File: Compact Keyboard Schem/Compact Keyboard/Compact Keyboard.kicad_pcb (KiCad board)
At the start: 2 copper layers, 105.5 x 115.1 mm, 35 parts, among them J1 MUX+POT, J2 MUX Power, J4 PAM8406 Power, J5 ILI 9341, J6 USB_A, J7 Rotary_Encoder, J8 USB_Host, J9 Jack-DC, Q1 Q_PMOS_GSD, Q2 Q_PMOS_GSD, SW1 SW_Push_LED, SW2 SW_Push, SW3 SW_Push, SW4 SW_Push, SW5 SW_Push

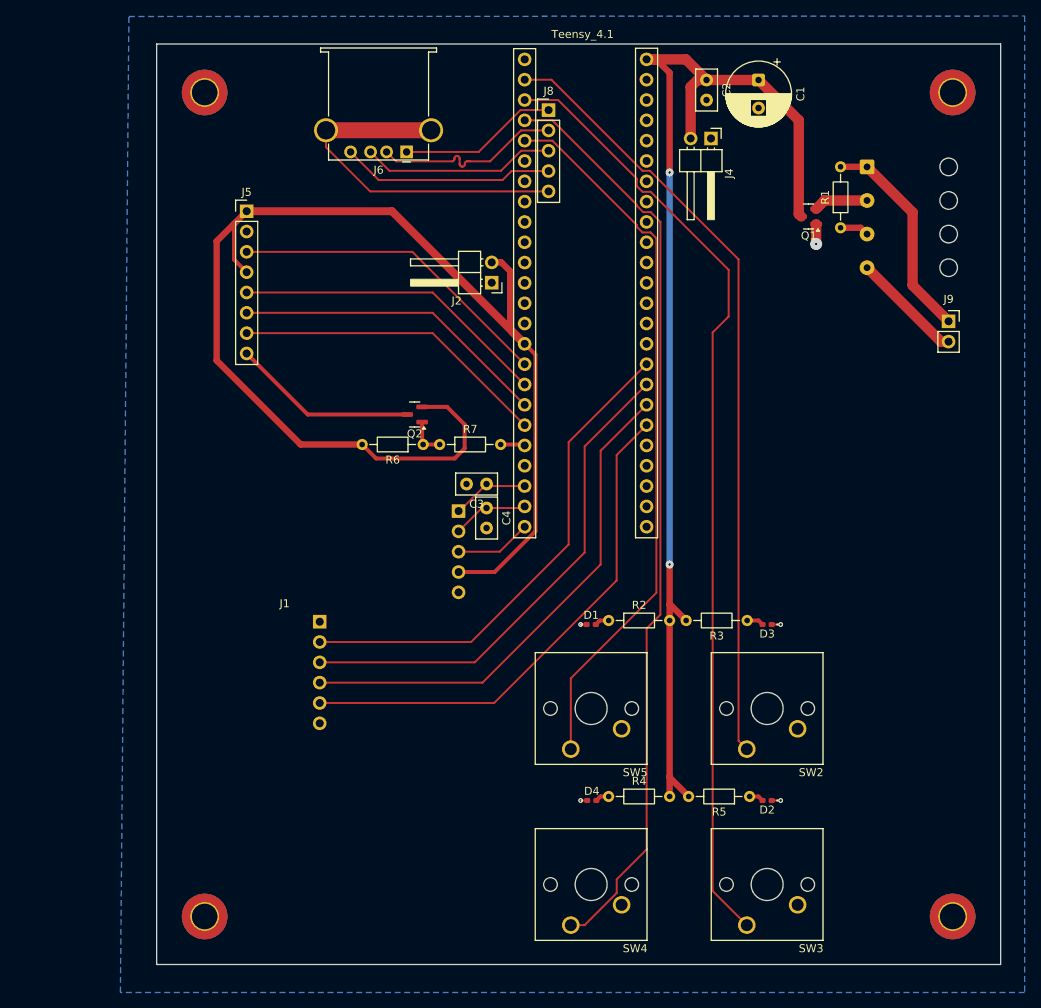
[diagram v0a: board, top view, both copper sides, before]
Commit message: Pushing Update
Latest version after PCB printing
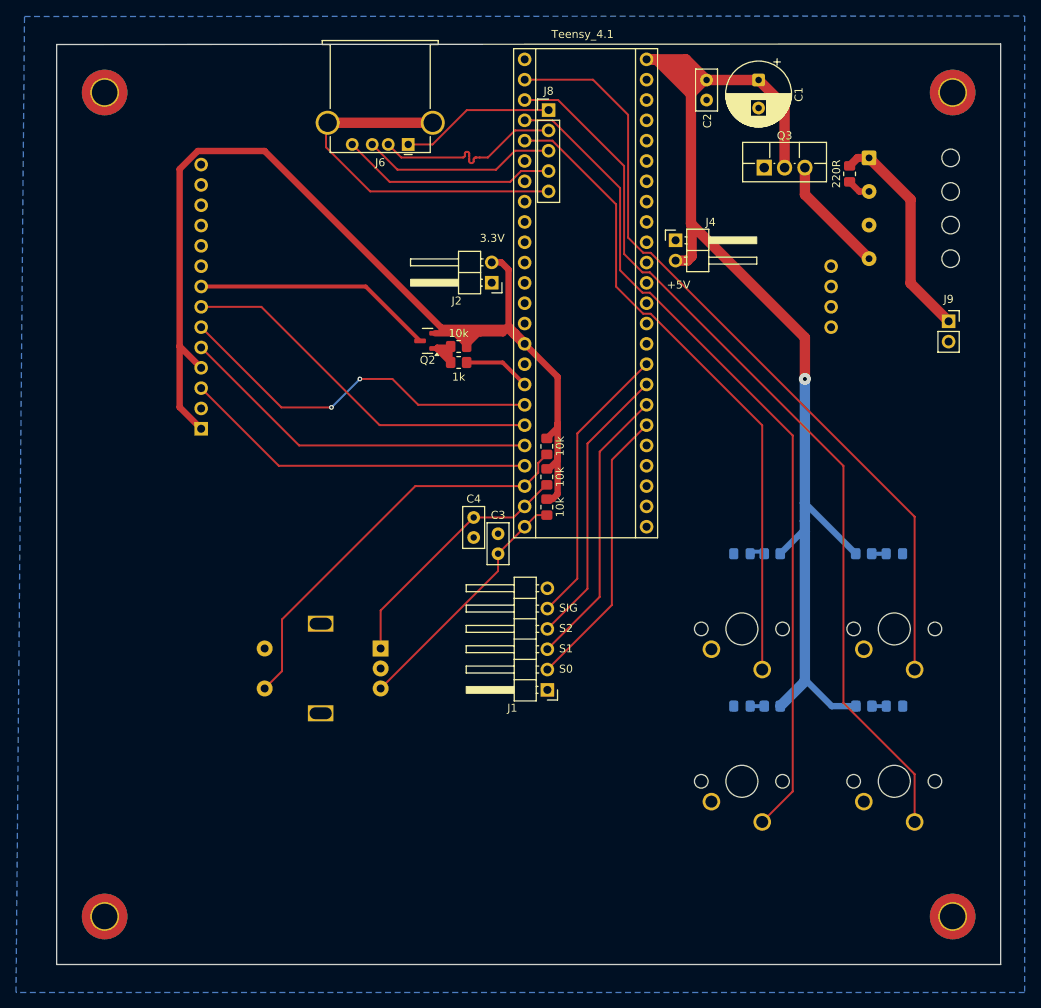
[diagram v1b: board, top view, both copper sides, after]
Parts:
- removed J5: ILI 9341, Connector_PinHeader_2.54mm:PinHeader_1x08_P2.54mm_Vertical
- removed J7: Rotary_Encoder, Connector_PinHeader_2.54mm:PinHeader_1x05_P2.54mm_Horizontal
- removed Q1: Q_PMOS_GSD, Package_TO_SOT_SMD:SOT-23
- added 10k: 10K, Resistor_SMD:R_0805_2012Metric_Pad1.20x1.40mm_HandSolder, F.Cu at (144.3, 83.3)
- added 10k: 10K, Resistor_SMD:R_0805_2012Metric_Pad1.20x1.40mm_HandSolder, F.Cu at (144.3, 79.5)
- added 10k: 10K, Resistor_SMD:R_0805_2012Metric_Pad1.20x1.40mm_HandSolder, F.Cu at (144.3, 75.7)
- added J3: SW_Switch_LED, Connector_Wire:SolderWire-0.25sqmm_1x04_P4.2mm_D0.65mm_OD1.7mm_Relief, B.Cu at (184.5, 39.7)
- added Q3: Q_PMOS_GDS, Package_TO_SOT_THT:TO-220F-3_Vertical, F.Cu at (171.5, 40.9)
- added TFT_ILI1: ~, TOMD:ILI9341_TFT, B.Cu at (140.4, 40.5)
- 10k: renamed from R6; footprint Resistor_THT:R_Axial_DIN0204_L3.6mm_D1.6mm_P7.62mm_Horizontal -> Resistor_SMD:R_0805_2012Metric_Pad1.20x1.40mm_HandSolder
- 1k: renamed from R7; footprint Resistor_THT:R_Axial_DIN0204_L3.6mm_D1.6mm_P7.62mm_Horizontal -> Resistor_SMD:R_0805_2012Metric_Pad1.20x1.40mm_HandSolder
- 220R: renamed from R1; footprint Resistor_THT:R_Axial_DIN0204_L3.6mm_D1.6mm_P7.62mm_Horizontal -> Resistor_SMD:R_0805_2012Metric_Pad1.20x1.40mm_HandSolder
- 220R: renamed from R5; footprint Resistor_THT:R_Axial_DIN0204_L3.6mm_D1.6mm_P7.62mm_Horizontal -> Resistor_SMD:R_0805_2012Metric_Pad1.20x1.40mm_HandSolder; moved to B.Cu
- 220R: renamed from R4; footprint Resistor_THT:R_Axial_DIN0204_L3.6mm_D1.6mm_P7.62mm_Horizontal -> Resistor_SMD:R_0805_2012Metric_Pad1.20x1.40mm_HandSolder; moved to B.Cu
- 220R: renamed from R2; footprint Resistor_THT:R_Axial_DIN0204_L3.6mm_D1.6mm_P7.62mm_Horizontal -> Resistor_SMD:R_0805_2012Metric_Pad1.20x1.40mm_HandSolder; moved to B.Cu
- 220R: renamed from R3; footprint Resistor_THT:R_Axial_DIN0204_L3.6mm_D1.6mm_P7.62mm_Horizontal -> Resistor_SMD:R_0805_2012Metric_Pad1.20x1.40mm_HandSolder; moved to B.Cu
- D1, D2, D3, D4: footprint LED_SMD:LED_0402_1005Metric_Pad0.77x0.64mm_HandSolder -> LED_SMD:LED_0805_2012Metric_Pad1.15x1.40mm_HandSolder; moved to B.Cu
- J1: moved to F.Cu
- SW1: value SW_Push_LED -> RotaryEncoder_Switch_MP; footprint Connector_Wire:SolderWire-0.25sqmm_1x04_P4.2mm_D0.65mm_OD1.7mm_Relief -> Rotary_Encoder:RotaryEncoder_Alps_EC11E-Switch_Vertical_H20mm
- SW2, SW3, SW4, SW5: moved to B.Cu
- moved SW1 85.6 mm to (123.5, 101.0), turned to 180 degrees
- moved D4 39.6 mm to (187.7, 108.2), turned to 180 degrees
- moved D1 38.9 mm to (187.7, 89.2), turned to 180 degrees
- moved 220R 33.9 mm to (183.9, 108.2), turned to 180 degrees
- moved 220R 33.0 mm to (183.9, 89.2), turned to 180 degrees
- moved J1 29.7 mm to (144.3, 106.2)
- moved SW4 27.2 mm to (171.2, 122.7), turned to 0 degrees
- moved SW5 25.9 mm to (171.2, 103.6), turned to 0 degrees
- moved SW3 24.6 mm to (190.2, 122.7), turned to 0 degrees
- moved SW2 23.2 mm to (190.2, 103.6), turned to 0 degrees
- moved J4 13.5 mm to (160.4, 50.0), turned to 0 degrees
- moved 10k 13.0 mm to (133.2, 63.2), turned to 0 degrees
- moved REF** 12.5 mm to (89.0, 31.5)
- moved REF** 12.5 mm to (89.0, 134.5)
- moved D2 12.2 mm to (168.7, 108.2), turned to 0 degrees
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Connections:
- 220R pad 1: Net-(SW1-K) -> Net-(J3-Pin_2)
- 220R pad 2: Net-(J9-Pad1) -> Net-(J3-Pin_1)
- J1 pad 2: /SIG_MUX -> /S0_MUX
- J1 pad 3: /S2_MUX -> /S1_MUX
- J1 pad 4: /S1_MUX -> /S2_MUX
- J1 pad 5: /S0_MUX -> /SIG_MUX
- J9 pad 1: Net-(J9-Pad1) -> Net-(J3-Pin_1)
- Teensy_4.1 pad 16: /ILI_9341/CS_LCD -> unconnected-(Teensy_4.1-24-Pad16)
- Teensy_4.1 pad 17: /ILI_9341/DC_LCD -> /ILI_9341/LED_LCD
- Teensy_4.1 pad 20: /ILI_9341/LED_LCD -> /ILI_9341/DC_LCD
- Teensy_4.1 pad 21: unconnected-(Teensy_4.1-29-Pad21) -> /ILI_9341/CS_LCD
- Teensy_4.1 pad 22: /Rotary_Encoder/CLK_RE -> /Rotary_Encoder/SW_RE
- Teensy_4.1 pad 24: /Rotary_Encoder/SW_RE -> /Rotary_Encoder/CLK_RE
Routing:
- net /Rotary_Encoder/SW_RE: track 9.55 -> 51.9 mm
- net /S0_MUX: track 64.4 -> 35.7 mm
- net /S1_MUX: track 63.6 -> 35.7 mm
- net Net-(J3-Pin_1): track 0.00 -> 27.4 mm
- net /S2_MUX: track 63.0 -> 35.7 mm
- net /SIG_MUX: track 62.7 -> 35.7 mm
- net Net-(J9-Pad1): track 26.8 -> 0.00 mm
- net +3.3V: track 164.9 -> 142.2 mm
- net /Rotary_Encoder/DT_RE: track 9.55 -> 32.0 mm
- net /Rotary_Encoder/CLK_RE: track 9.77 -> 31.0 mm
- net GND: track 20.3 -> 0.00 mm, vias 5 -> 0
- net Net-(J3-Pin_4): track 0.00 -> 14.7 mm
- net /Buttons/BTN3_IN: track 115.8 -> 105.7 mm
- net /Buttons/BTN4_IN: track 89.9 -> 81.0 mm
- net /ILI_9341/MOSI_LCD: track 39.5 -> 47.4 mm, vias 0 -> 2
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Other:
- board size 105.5 x 115.1 mm -> 118 x 115.1 mm
- board text added: "+5V"
- board text added: "3.3V"
- board text added: "S0"
- board text added: "S1"
- board text added: "S2"
- board text added: "SIG"
